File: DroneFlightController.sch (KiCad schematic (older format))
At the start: 11 parts, among them J1 USB_B_Micro, U1 STM32H743VITx, Y1 CSTNE8M00G550000R0

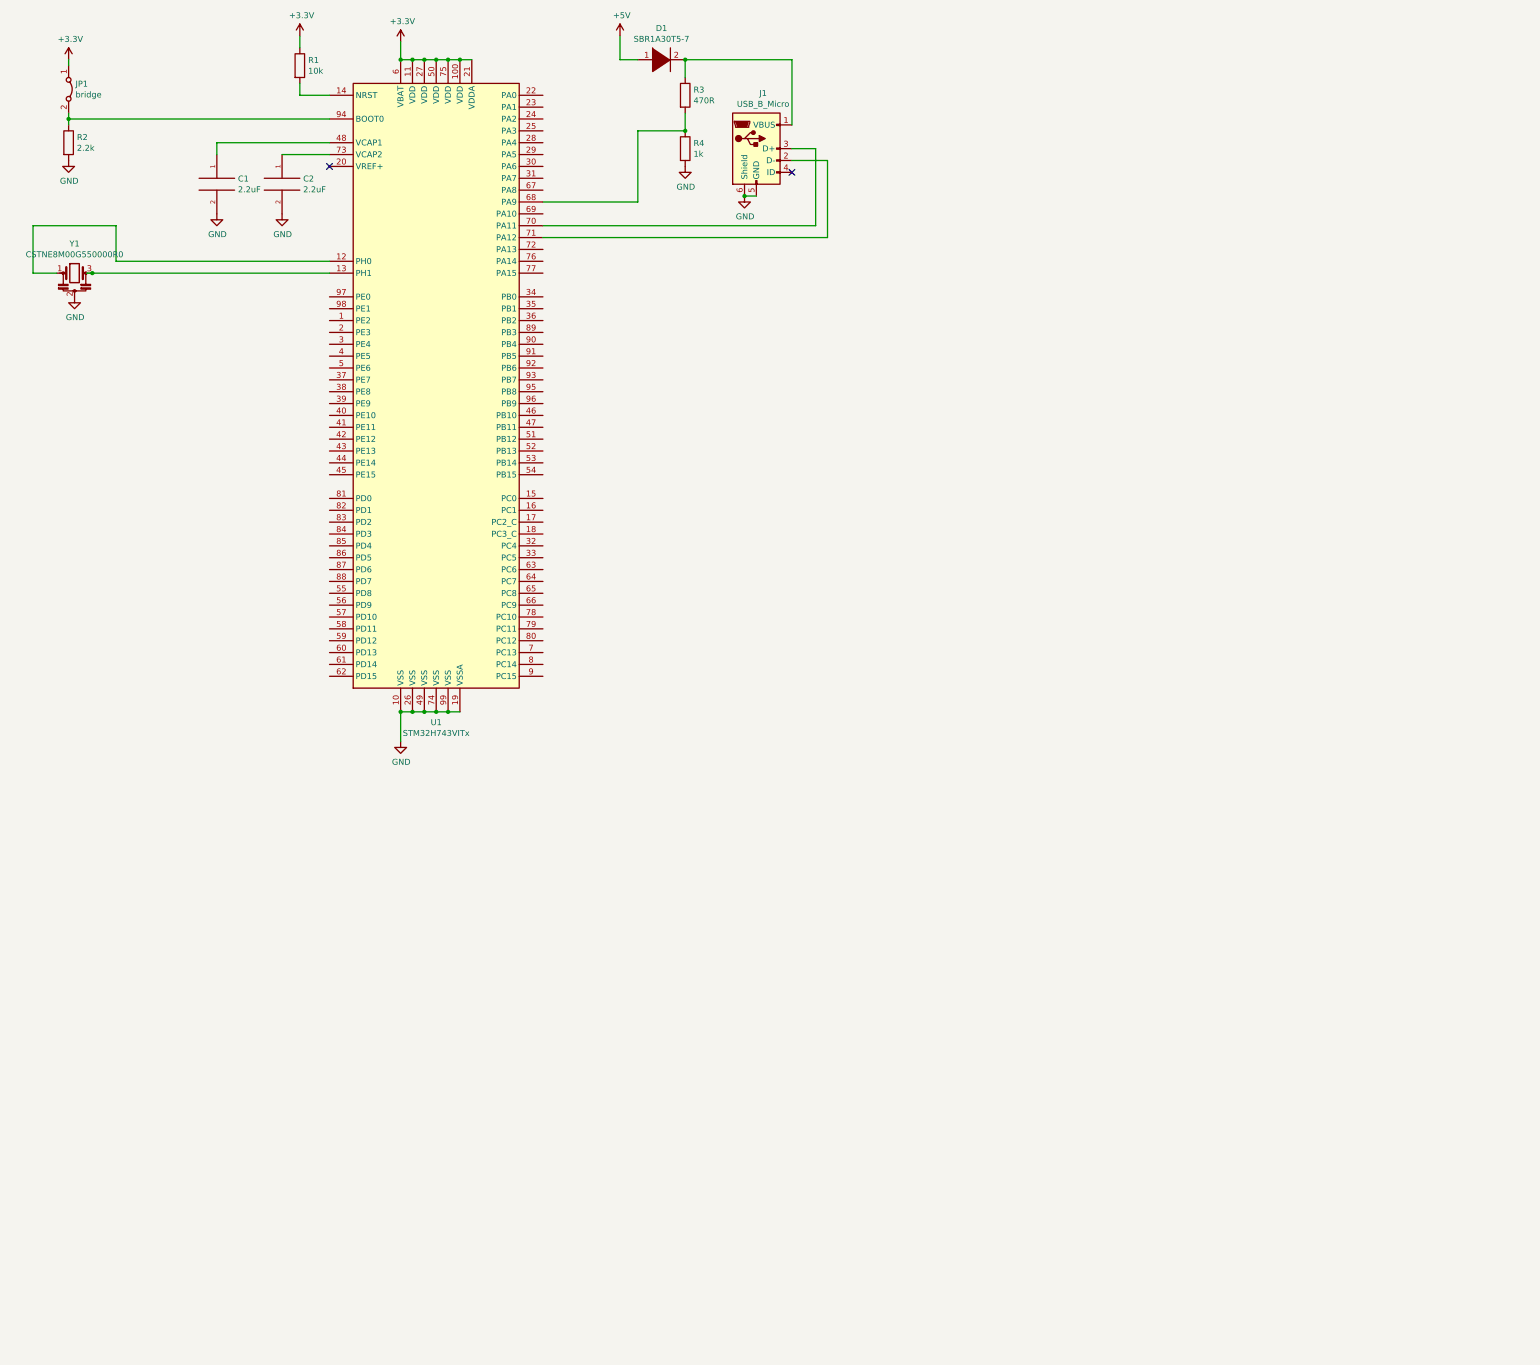
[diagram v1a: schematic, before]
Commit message: I may have fucked up...
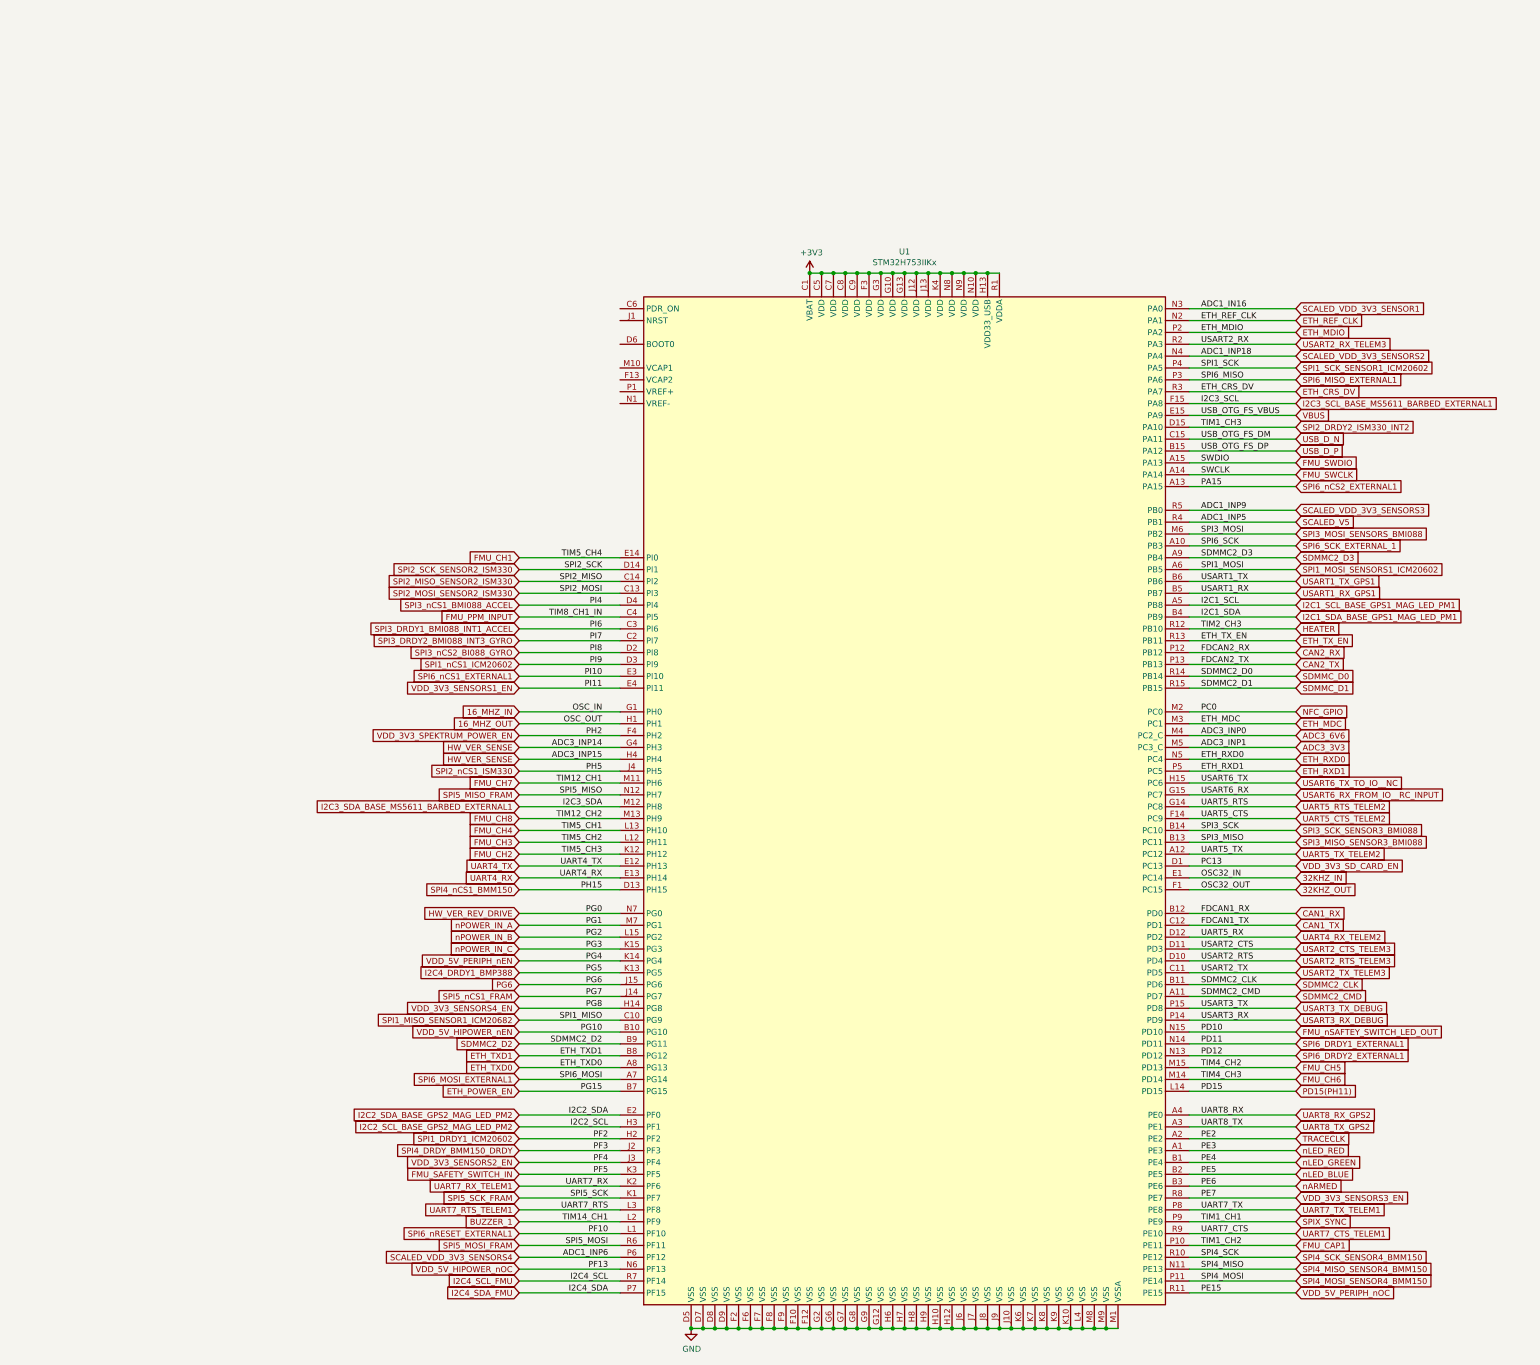
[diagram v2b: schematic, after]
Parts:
- removed C1, C2: 2.2uF, symbol pspice:C
- removed D1: SBR1A30T5-7, symbol pspice:DIODE
- removed J1: USB_B_Micro, symbol Connector:USB_B_Micro
- removed JP1: bridge, symbol Jumper:Jumper_2_Bridged
- removed R1: 10k, symbol Device:R
- removed R2: 2.2k, symbol Device:R
- removed R3: 470R, symbol Device:R
- removed R4: 1k, symbol Device:R
- removed U1: STM32H743VITx, Package_QFP:LQFP-100_14x14mm_P0.5mm, symbol MCU_ST_STM32H7:STM32H743VITx
- removed Y1: CSTNE8M00G550000R0, symbol Device:Resonator
- added U1: STM32H753IIKx, Package_BGA:UFBGA-201_10x10mm_Layout15x15_P0.65mm, symbol MCU_ST_STM32H7:STM32H753IIKx
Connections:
- net +3V3: now also U1.C1 (VBAT), U1.C5 (VDD), U1.C7 (VDD), U1.C8 (VDD), U1.C9 (VDD), U1.F3 (VDD), U1.G10 (VDD), U1.G13 (VDD), U1.G3 (VDD), U1.H13 (VDD33_USB), U1.J12 (VDD), U1.J13 (VDD), U1.K4 (VDD), U1.N10 (VDD), U1.N8 (VDD), U1.N9 (VDD), U1.R1 (VDDA)
- net GND: now also U1.D5 (VSS), U1.D7 (VSS), U1.D8 (VSS), U1.D9 (VSS), U1.F10 (VSS), U1.F12 (VSS), U1.F2 (VSS), U1.F6 (VSS), U1.F7 (VSS), U1.F8 (VSS), U1.F9 (VSS), U1.G12 (VSS), U1.G2 (VSS), U1.G6 (VSS), U1.G7 (VSS), U1.G8 (VSS), U1.G9 (VSS), U1.H10 (VSS), U1.H12 (VSS), U1.H6 (VSS), U1.H7 (VSS), U1.H8 (VSS), U1.H9 (VSS), U1.J10 (VSS), U1.J6 (VSS), U1.J7 (VSS), U1.J8 (VSS), U1.J9 (VSS), U1.K10 (VSS), U1.K6 (VSS), U1.K7 (VSS), U1.K8 (VSS), U1.K9 (VSS), U1.L4 (VSS), U1.M1 (VSSA), U1.M8 (VSS), U1.M9 (VSS)
- new net 16_MHZ_IN: U1.G1 (PH0)
- new net 16_MHZ_OUT: U1.H1 (PH1)
- new net 32KHZ_IN: U1.E1 (PC14)
- new net 32KHZ_OUT: U1.F1 (PC15)
- new net ADC3_3V3: U1.M5 (PC3_C)
- new net ADC3_6V6: U1.M4 (PC2_C)
- new net BUZZER_1: U1.L2 (PF9)
- new net CAN1_RX: U1.B12 (PD0)
- new net CAN1_TX: U1.C12 (PD1)
- new net CAN2_RX: U1.P12 (PB12)
- new net CAN2_TX: U1.P13 (PB13)
- new net ETH_CRS_DV: U1.R3 (PA7)
- new net ETH_MDC: U1.M3 (PC1)
- new net ETH_MDIO: U1.P2 (PA2)
- new net ETH_POWER_EN: U1.B7 (PG15)
- new net ETH_REF_CLK: U1.N2 (PA1)
- new net ETH_RXD0: U1.N5 (PC4)
- new net ETH_RXD1: U1.P5 (PC5)
- new net ETH_TXD0: U1.A8 (PG13)
- new net ETH_TXD1: U1.B8 (PG12)
- new net ETH_TX_EN: U1.R13 (PB11)
- new net FMU_CAP1: U1.P10 (PE11)
- new net FMU_CH1: U1.E14 (PI0)
- new net FMU_CH2: U1.K12 (PH12)
- new net FMU_CH3: U1.L12 (PH11)
- new net FMU_CH4: U1.L13 (PH10)
- new net FMU_CH5: U1.M15 (PD13)
- new net FMU_CH6: U1.M14 (PD14)
- new net FMU_CH7: U1.M11 (PH6)
- new net FMU_CH8: U1.M13 (PH9)
- new net FMU_PPM_INPUT: U1.C4 (PI5)
- new net FMU_SAFETY_SWITCH_IN: U1.K3 (PF5)
- new net FMU_SWCLK: U1.A14 (PA14)
- new net FMU_SWDIO: U1.A15 (PA13)
- new net FMU_nSAFTEY_SWITCH_LED_OUT: U1.N15 (PD10)
- new net HEATER: U1.R12 (PB10)
- new net HW_VER_REV_DRIVE: U1.N7 (PG0)
- new net HW_VER_SENSE: U1.G4 (PH3), U1.H4 (PH4)
- new net I2C1_SCL_BASE_GPS1_MAG_LED_PM1: U1.A5 (PB8)
- new net I2C1_SDA_BASE_GPS1_MAG_LED_PM1: U1.B4 (PB9)
- new net I2C2_SCL_BASE_GPS2_MAG_LED_PM2: U1.H3 (PF1)
- new net I2C2_SDA_BASE_GPS2_MAG_LED_PM2: U1.E2 (PF0)
- new net I2C3_SCL_BASE_MS5611_BARBED_EXTERNAL1: U1.F15 (PA8)
- new net I2C3_SDA_BASE_MS5611_BARBED_EXTERNAL1: U1.M12 (PH8)
- new net I2C4_DRDY1_BMP388: U1.K13 (PG5)
- new net I2C4_SCL_FMU: U1.R7 (PF14)
- new net I2C4_SDA_FMU: U1.P7 (PF15)
- new net NFC_GPIO: U1.M2 (PC0)
- new net PD15(PH11): U1.L14 (PD15)
- new net PG6: U1.J15 (PG6)
- new net SCALED_V5: U1.R4 (PB1)
- new net SCALED_VDD_3V3_SENSOR1: U1.N3 (PA0)
- new net SCALED_VDD_3V3_SENSORS2: U1.N4 (PA4)
- new net SCALED_VDD_3V3_SENSORS3: U1.R5 (PB0)
- new net SCALED_VDD_3V3_SENSORS4: U1.P6 (PF12)
- new net SDMMC2_CLK: U1.B11 (PD6)
- new net SDMMC2_CMD: U1.A11 (PD7)
- new net SDMMC2_D2: U1.B9 (PG11)
- new net SDMMC2_D3: U1.A9 (PB4)
- new net SDMMC_D0: U1.R14 (PB14)
- new net SDMMC_D1: U1.R15 (PB15)
- new net SPI1_DRDY1_ICM20602: U1.H2 (PF2)
- new net SPI1_MISO_SENSOR1_ICM20682: U1.C10 (PG9)
- new net SPI1_MOSI_SENSORS1_ICM20602: U1.A6 (PB5)
- new net SPI1_SCK_SENSOR1_ICM20602: U1.P4 (PA5)
- new net SPI1_nCS1_ICM20602: U1.D3 (PI9)
- new net SPI2_DRDY2_ISM330_INT2: U1.D15 (PA10)
- new net SPI2_MISO_SENSOR2_ISM330: U1.C14 (PI2)
- new net SPI2_MOSI_SENSOR2_ISM330: U1.C13 (PI3)
- new net SPI2_SCK_SENSOR2_ISM330: U1.D14 (PI1)
- new net SPI2_nCS1_ISM330: U1.J4 (PH5)
- new net SPI3_DRDY1_BMI088_INT1_ACCEL: U1.C3 (PI6)
- new net SPI3_DRDY2_BMI088_INT3_GYRO: U1.C2 (PI7)
- new net SPI3_MISO_SENSOR3_BMI088: U1.B13 (PC11)
- new net SPI3_MOSI_SENSORS_BMI088: U1.M6 (PB2)
- new net SPI3_SCK_SENSOR3_BMI088: U1.B14 (PC10)
- new net SPI3_nCS1_BMI088_ACCEL: U1.D4 (PI4)
- new net SPI3_nCS2_BI088_GYRO: U1.D2 (PI8)
- new net SPI4_DRDY_BMM150_DRDY: U1.J2 (PF3)
- new net SPI4_MISO_SENSOR4_BMM150: U1.N11 (PE13)
- new net SPI4_MOSI_SENSOR4_BMM150: U1.P11 (PE14)
- new net SPI4_SCK_SENSOR4_BMM150: U1.R10 (PE12)
- new net SPI4_nCS1_BMM150: U1.D13 (PH15)
- new net SPI5_MISO_FRAM: U1.N12 (PH7)
- new net SPI5_MOSI_FRAM: U1.R6 (PF11)
- new net SPI5_SCK_FRAM: U1.K1 (PF7)
- new net SPI5_nCS1_FRAM: U1.J14 (PG7)
- new net SPI6_DRDY1_EXTERNAL1: U1.N14 (PD11)
- new net SPI6_DRDY2_EXTERNAL1: U1.N13 (PD12)
- new net SPI6_MISO_EXTERNAL1: U1.P3 (PA6)
- new net SPI6_MOSI_EXTERNAL1: U1.A7 (PG14)
- new net SPI6_SCK_EXTERNAL_1: U1.A10 (PB3)
- new net SPI6_nCS1_EXTERNAL1: U1.E3 (PI10)
- new net SPI6_nCS2_EXTERNAL1: U1.A13 (PA15)
- new net SPI6_nRESET_EXTERNAL1: U1.L1 (PF10)
- new net SPIX_SYNC: U1.P9 (PE9)
- new net TRACECLK: U1.A2 (PE2)
- new net UART4_RX: U1.E13 (PH14)
- new net UART4_RX_TELEM2: U1.D12 (PD2)
- new net UART4_TX: U1.E12 (PH13)
- new net UART5_CTS_TELEM2: U1.F14 (PC9)
- new net UART5_RTS_TELEM2: U1.G14 (PC8)
- new net UART5_TX_TELEM2: U1.A12 (PC12)
- new net UART7_CTS_TELEM1: U1.R9 (PE10)
- new net UART7_RTS_TELEM1: U1.L3 (PF8)
- new net UART7_RX_TELEM1: U1.K2 (PF6)
- new net UART7_TX_TELEM1: U1.P8 (PE8)
- new net UART8_RX_GPS2: U1.A4 (PE0)
- new net UART8_TX_GPS2: U1.A3 (PE1)
- new net USART1_RX_GPS1: U1.B5 (PB7)
- new net USART1_TX_GPS1: U1.B6 (PB6)
- new net USART2_CTS_TELEM3: U1.D11 (PD3)
- new net USART2_RTS_TELEM3: U1.D10 (PD4)
- new net USART2_RX_TELEM3: U1.R2 (PA3)
- new net USART2_TX_TELEM3: U1.C11 (PD5)
- new net USART3_RX_DEBUG: U1.P14 (PD9)
- new net USART3_TX_DEBUG: U1.P15 (PD8)
- new net USART6_RX_FROM_IO__RC_INPUT: U1.G15 (PC7)
- new net USART6_TX_TO_IO__NC: U1.H15 (PC6)
- new net USB_D_N: U1.C15 (PA11)
- new net USB_D_P: U1.B15 (PA12)
- new net VBUS: U1.E15 (PA9)
- new net VDD_3V3_SD_CARD_EN: U1.D1 (PC13)
- new net VDD_3V3_SENSORS1_EN: U1.E4 (PI11)
- new net VDD_3V3_SENSORS2_EN: U1.J3 (PF4)
- new net VDD_3V3_SENSORS3_EN: U1.R8 (PE7)
- new net VDD_3V3_SENSORS4_EN: U1.H14 (PG8)
- new net VDD_3V3_SPEKTRUM_POWER_EN: U1.F4 (PH2)
- new net VDD_5V_HIPOWER_nEN: U1.B10 (PG10)
- new net VDD_5V_HIPOWER_nOC: U1.N6 (PF13)
- new net VDD_5V_PERIPH_nEN: U1.K14 (PG4)
- new net VDD_5V_PERIPH_nOC: U1.R11 (PE15)
- new net nARMED: U1.B3 (PE6)
- new net nLED_BLUE: U1.B2 (PE5)
- new net nLED_GREEN: U1.B1 (PE4)
- new net nLED_RED: U1.A1 (PE3)
- new net nPOWER_IN_A: U1.M7 (PG1)
- new net nPOWER_IN_B: U1.L15 (PG2)
- new net nPOWER_IN_C: U1.K15 (PG3)
- no-connect marks 2 -> 0
